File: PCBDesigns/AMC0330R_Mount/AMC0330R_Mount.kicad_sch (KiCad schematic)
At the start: 13 parts, among them J1 HV_Input, J2 Low_Side, U1 AMC0330R-Q1, U2 RFM-0505S

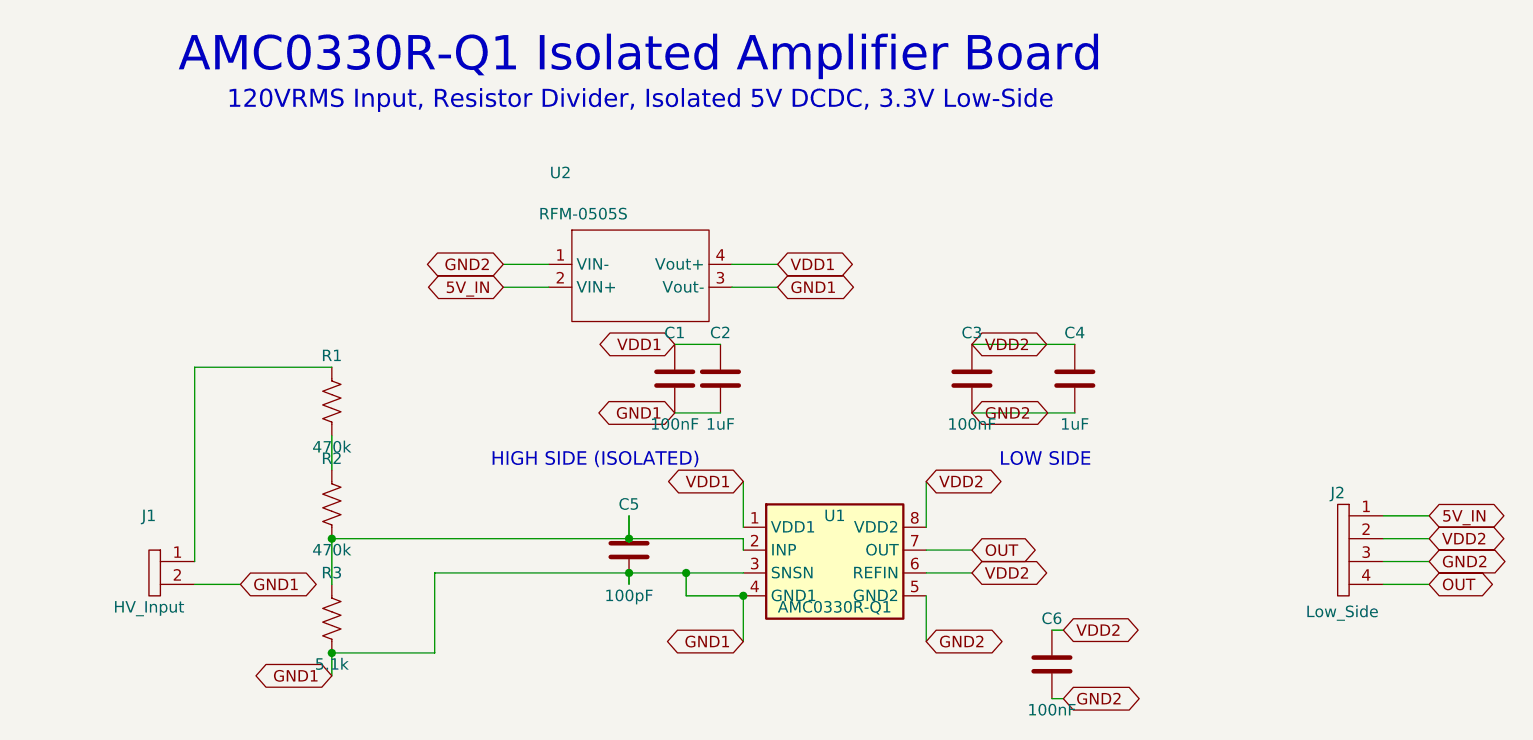
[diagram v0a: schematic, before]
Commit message: Various troubleshooting and PCB design
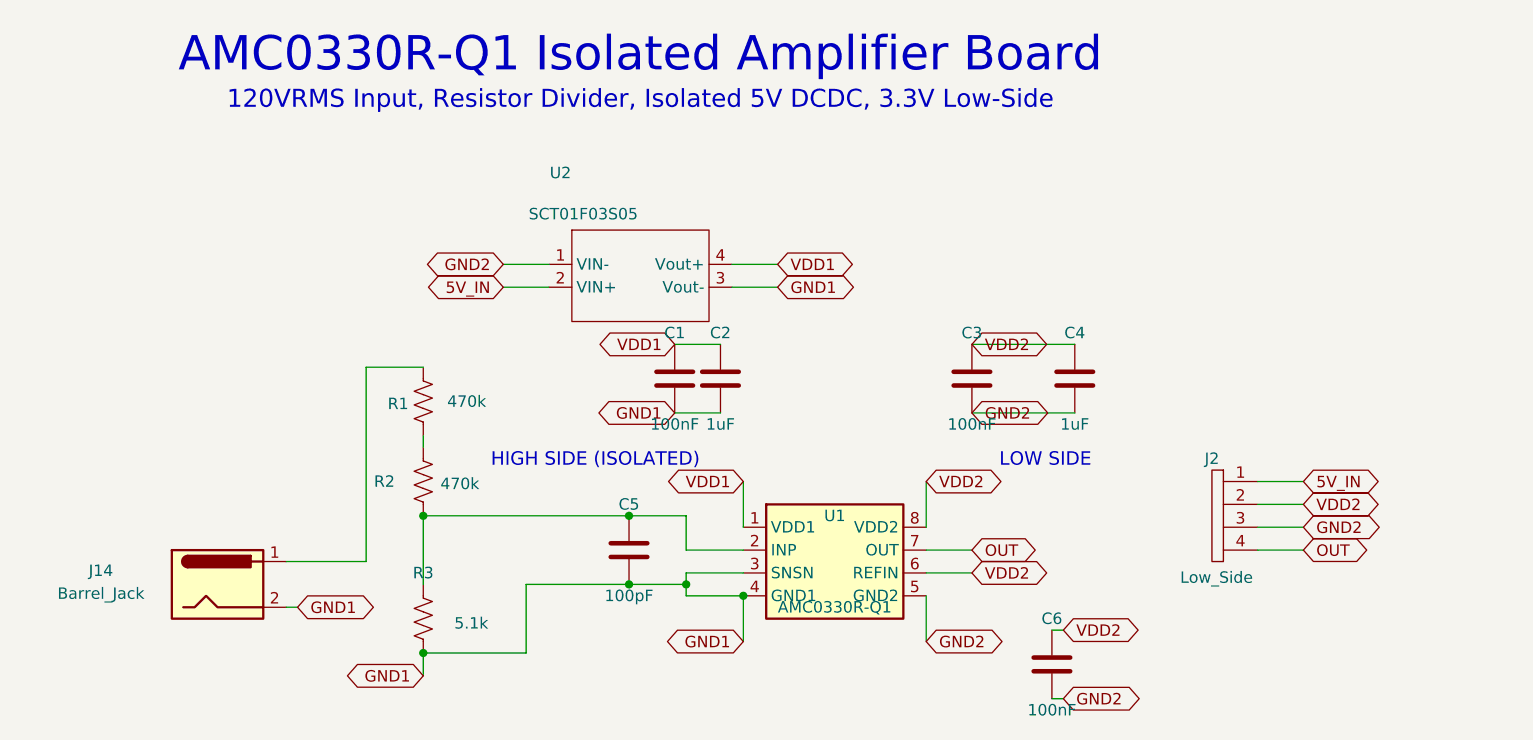
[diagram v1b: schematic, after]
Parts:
- removed J1: HV_Input, Connector_PinHeader_2.54mm:PinHeader_1x02_P2.54mm_Vertical, symbol Connector_Generic:Conn_01x02
- added J14: Barrel_Jack, Connector_BarrelJack:BarrelJack_Horizontal, symbol Connector:Barrel_Jack
- U2: value RFM-0505S -> SCT01F03S05
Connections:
- net GND1: now also J14.2
- net at R1.1: now also J14.1
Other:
- moved on the sheet: J2, R1, R2, R3
